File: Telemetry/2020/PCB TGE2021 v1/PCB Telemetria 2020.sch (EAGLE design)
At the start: 39 parts, among them IC1 INA240A1DR, IC2 MCP3221A6T-E_OTVAO, IC3 AZ1117IH-3.3TRG1, IC4 ACS758LCB-050B-PFF-T, IC5 ADS1115IDGSR, IC7 ACS758LCB-050B-PFF-T

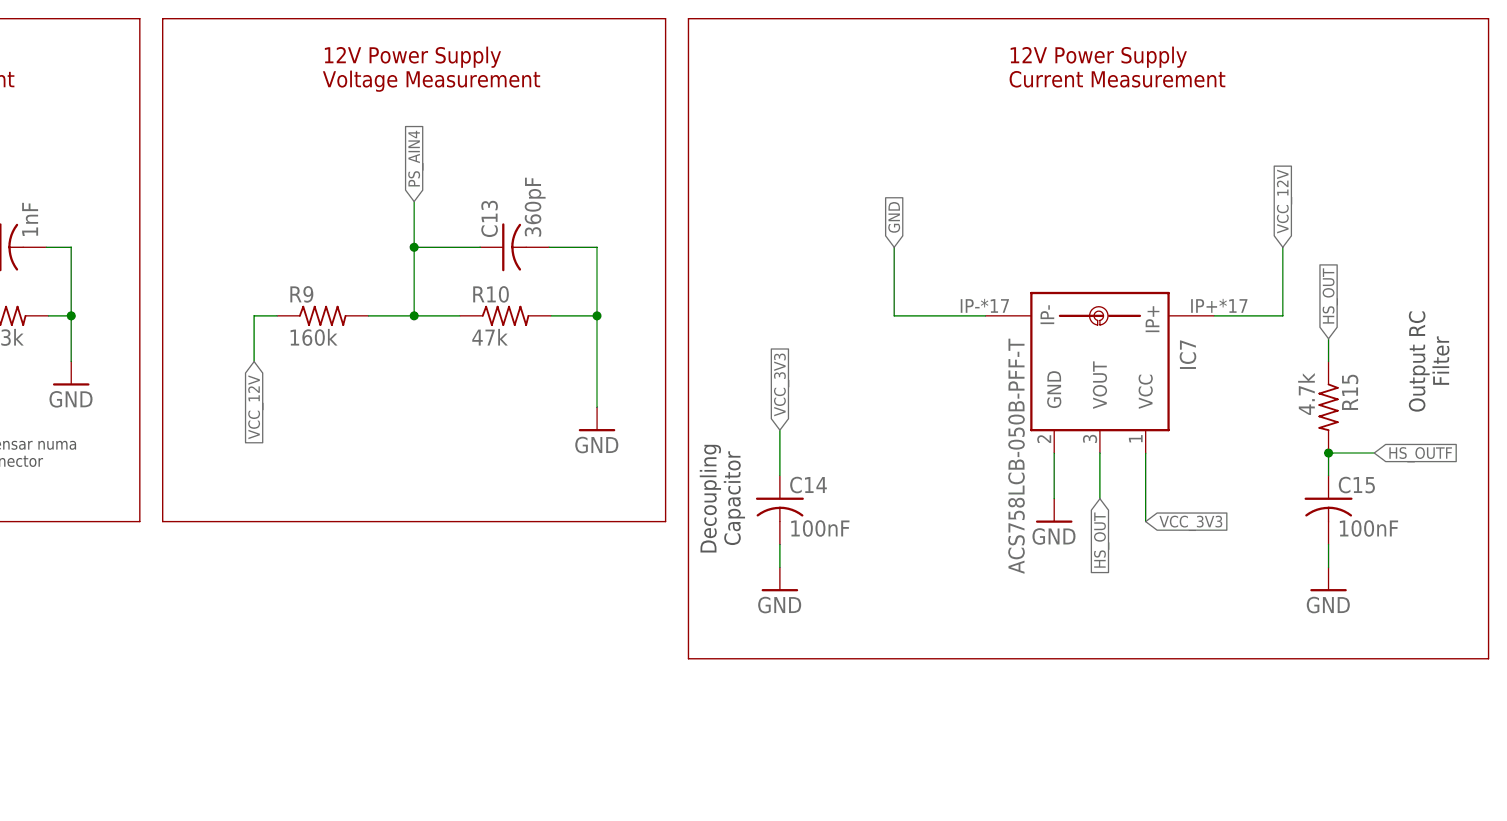
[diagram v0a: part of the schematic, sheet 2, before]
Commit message: corrigindo esquematico
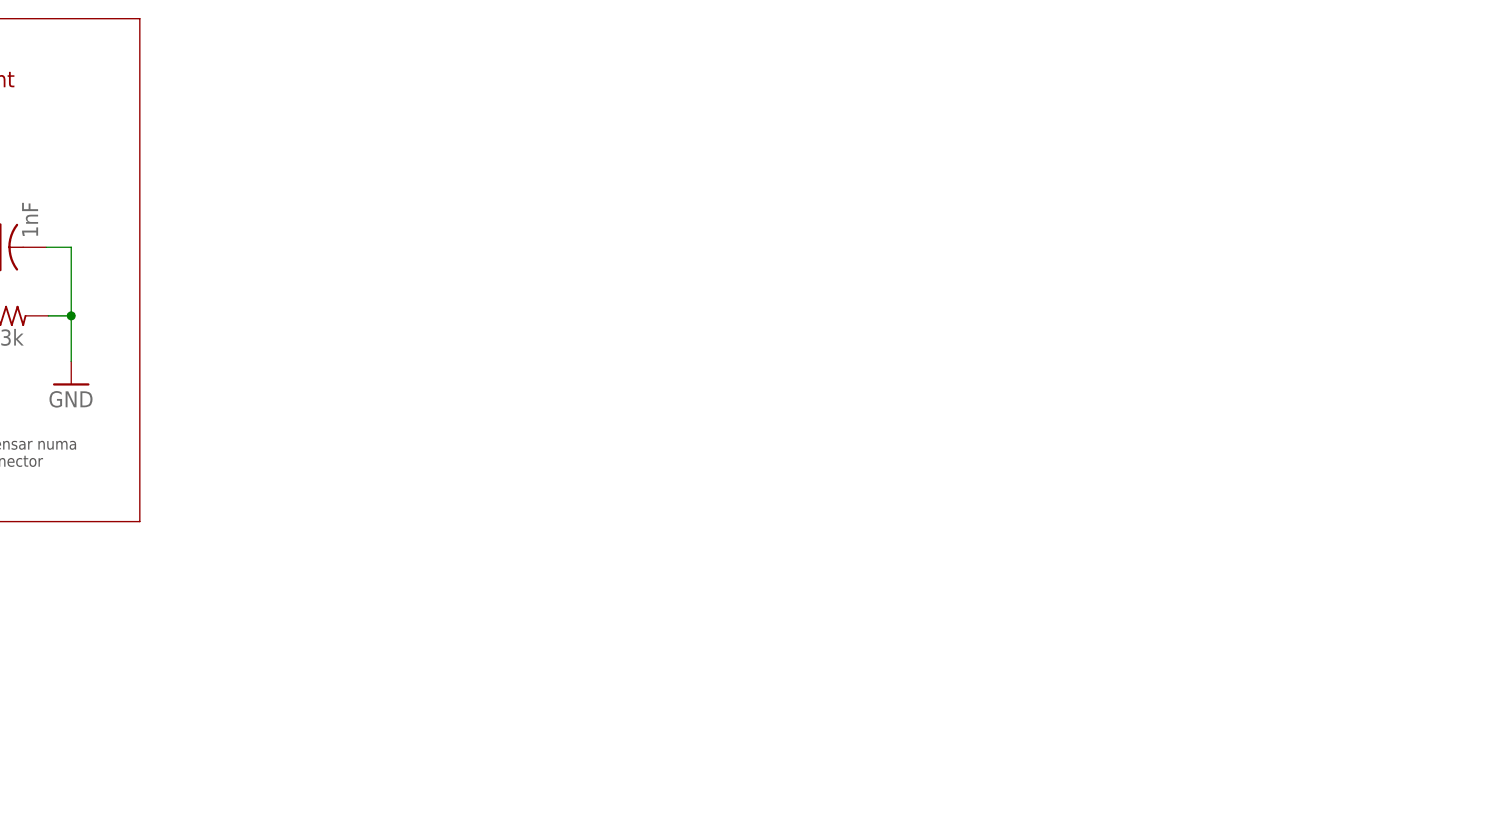
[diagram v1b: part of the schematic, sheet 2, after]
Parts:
- removed C13: 360pF, rcl:C-USC0805
- removed C14, C15: 100nF, rcl:C-USC0805
- removed IC7: ACS758LCB-050B-PFF-T, allegro:ACS758LCB-050B-PFF-T
- removed R10: 47k, rcl:R-US_R0805
- removed R15: 4.7k, rcl:R-US_R0805
- removed R9: 160k, rcl:R-US_R0805
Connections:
- removed net HS_OUT: IC7.VOUT, R15.1
- removed net HS_OUTF: C15.1, R15.2
- removed net PS_AIN4: C13.1, R10.1, R9.2
- net GND: no longer C13.2, C14.2, C15.2, IC7.GND, IC7.IP-, R10.2
- net VCC_12V: no longer IC7.IP+, R9.1
- net VCC_3V3: no longer C14.1, IC7.VCC
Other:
- note removed: "12V Power Supply Current Measurement"
- note removed: "12V Power Supply Voltage Measurement"
